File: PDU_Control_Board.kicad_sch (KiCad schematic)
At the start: 237 parts

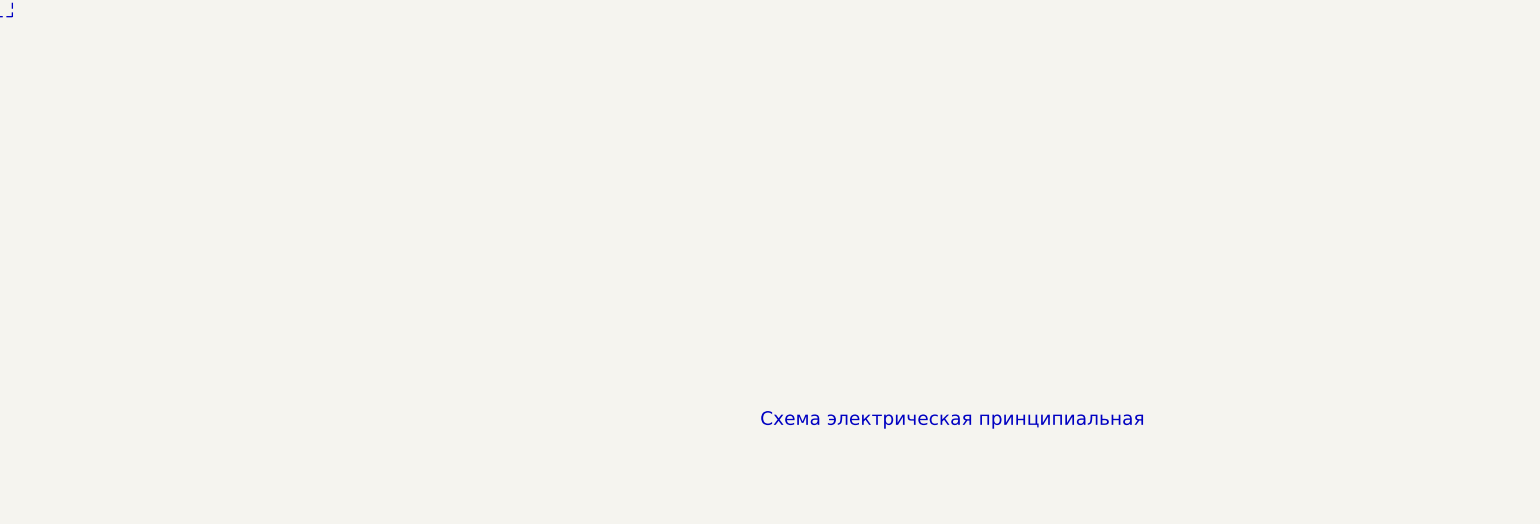
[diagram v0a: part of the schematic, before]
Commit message: VER1.1: переименовал Э3
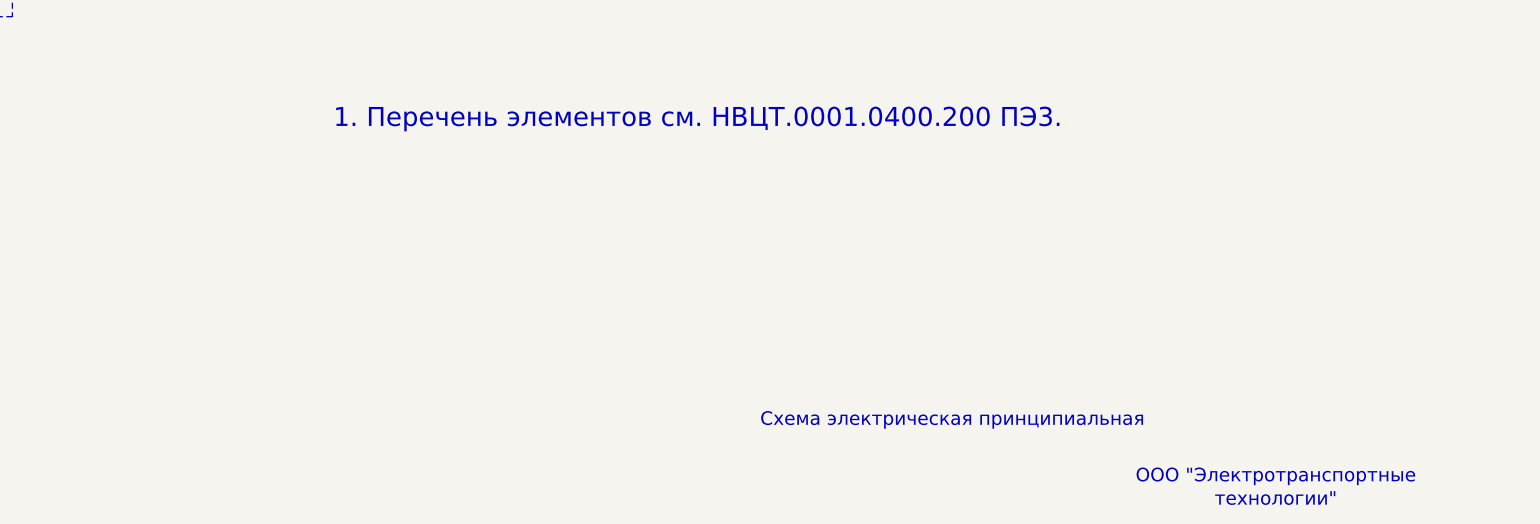
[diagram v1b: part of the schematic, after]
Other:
- note added: "1. Перечень элементов см. НВЦТ.0001.0400.200 ПЭ3."
- note added: "ООО "Электротранспортные"
- note added: "технологии""
- company: ООО "Электротранспортные технологии" -> (none)
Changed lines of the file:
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@@
 	(title_block
 		(title "Плата управления")
-		(company "ООО \"Электротранспортные технологии\"")
 		(comment 1 "НВЦТ.0001.0400.200 Э3")
 		(comment 2 "Филатов А.С.")
@@
 		)
 	)
+	(text "1. Перечень элементов см. НВЦТ.0001.0400.200 ПЭ3."
+		(exclude_from_sim no)
+		(at 704.342 512.826 0)
+		(effects
+			(font
+				(size 3.5 3.5)
+			)
+		)
+	)
 	(text "Питание 5В"
 		(exclude_from_sim no)
@@
 		)
 	)
+	(text "ООО \"Электротранспортные"
+		(exclude_from_sim no)
+		(at 811.022 578.866 0)
+		(effects
+			(font
+				(size 2.5 2.5)
+			)
+		)
+	)
+	(text "технологии\""
+		(exclude_from_sim no)
+		(at 811.022 583.184 0)
+		(effects
+			(font
+				(size 2.5 2.5)
+			)
+		)
+	)
